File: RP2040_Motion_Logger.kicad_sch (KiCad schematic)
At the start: 51 parts, among them J1 Conn_01x02, J3 TC2030-NL, P1 USB_C_Plug_USB2.0, Q1 AO3401A, SW1 RESET, U1 RP2040, U2 TLV62569DBV, U4 MCP73831-2-OT, Y1 12MHZ

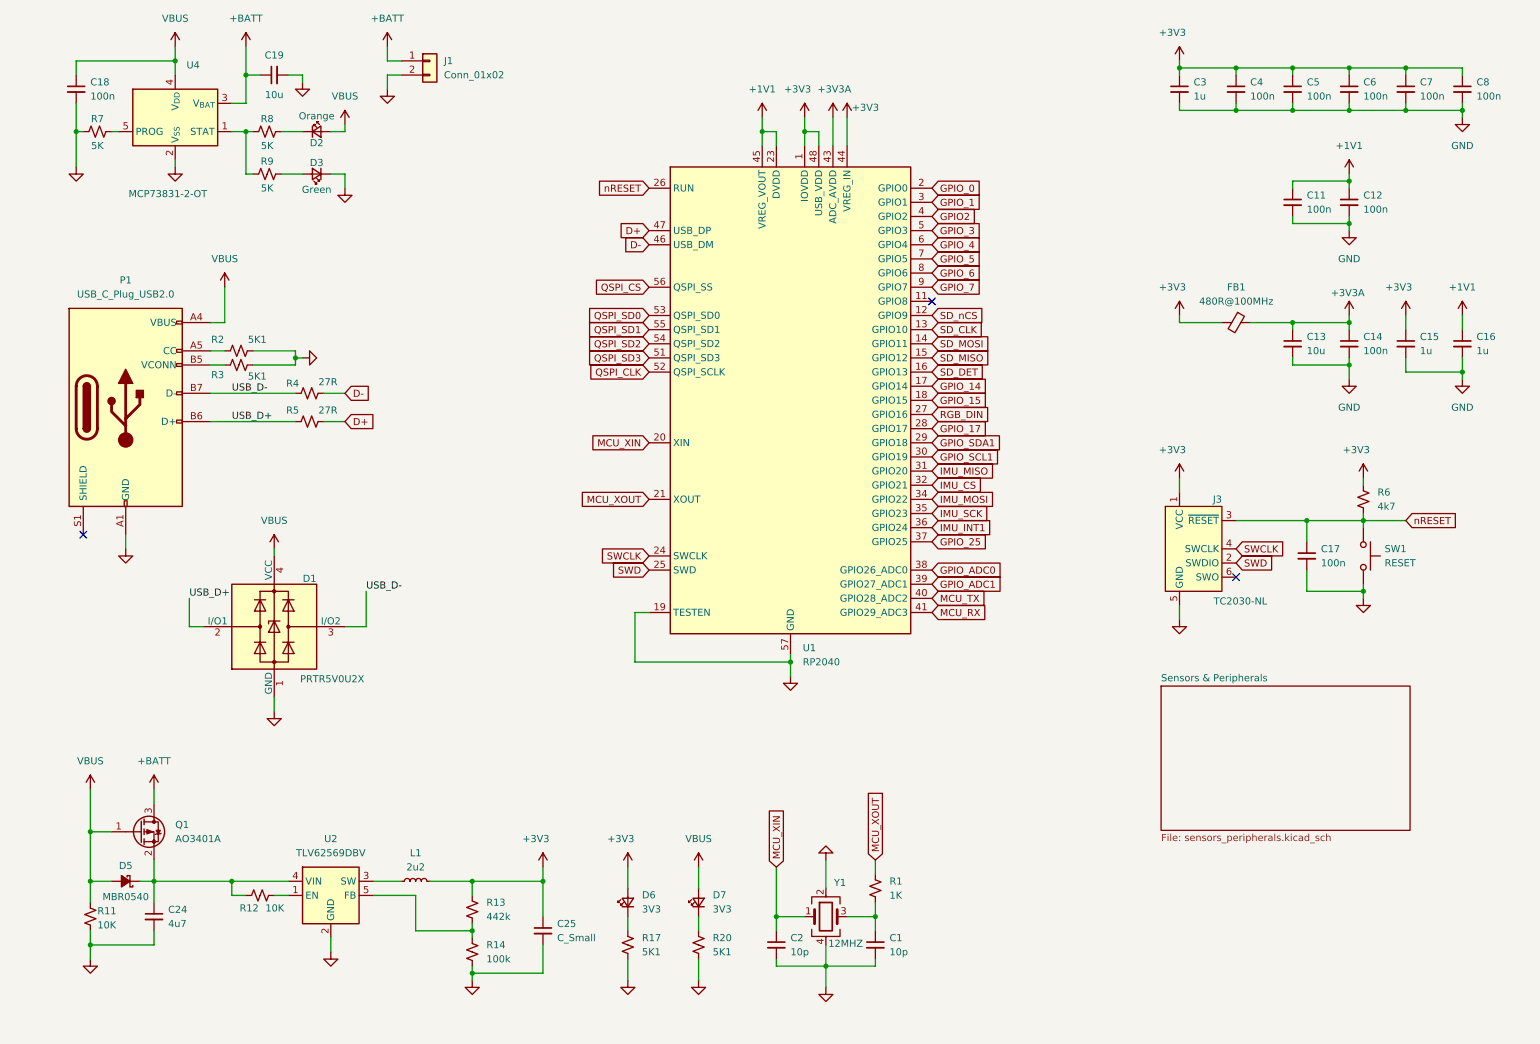
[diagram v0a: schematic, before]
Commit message: updated
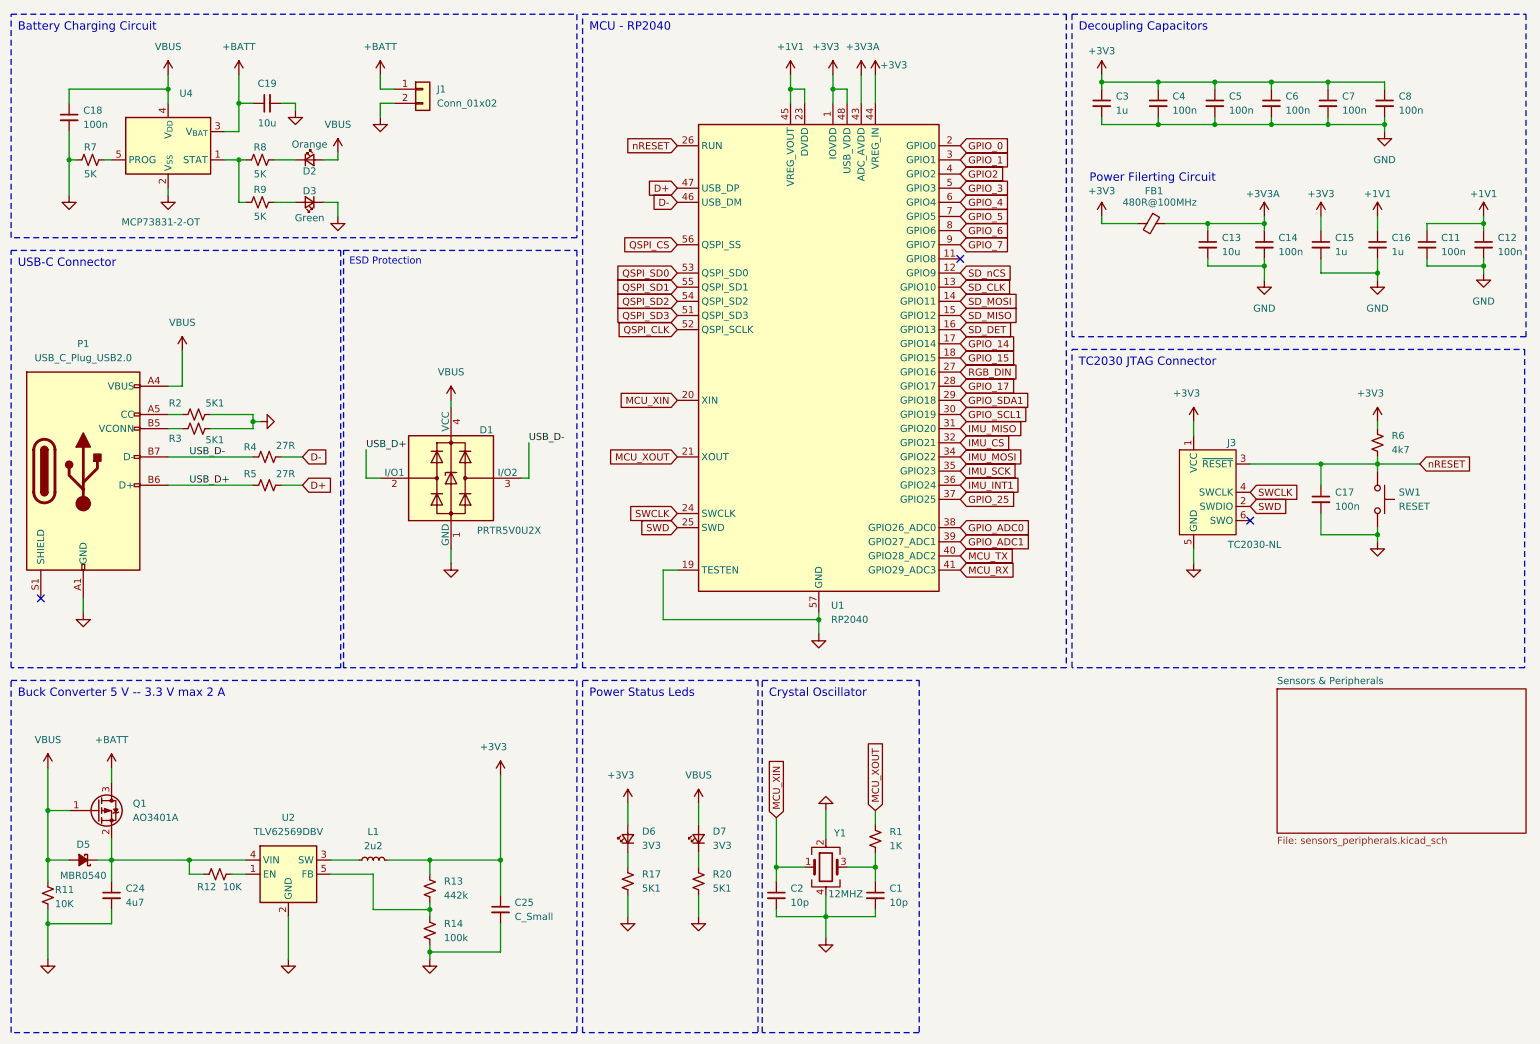
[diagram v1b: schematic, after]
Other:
- note added: "Power Filerting Circuit"
- company: (none) -> Rishikesh 
- title: (none) -> RP2040 Motion Logger
- moved on the sheet: C1, C11, C12, C13, C14, C15, C16, C17, C18, C19, C2, C24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
